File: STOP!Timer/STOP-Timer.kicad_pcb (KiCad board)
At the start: 2 copper layers, 4 parts, among them SW1 SW_Push_DPDT, U2 PEC11R-4230F-S0024, U3 PEC11R-4230F-S0024

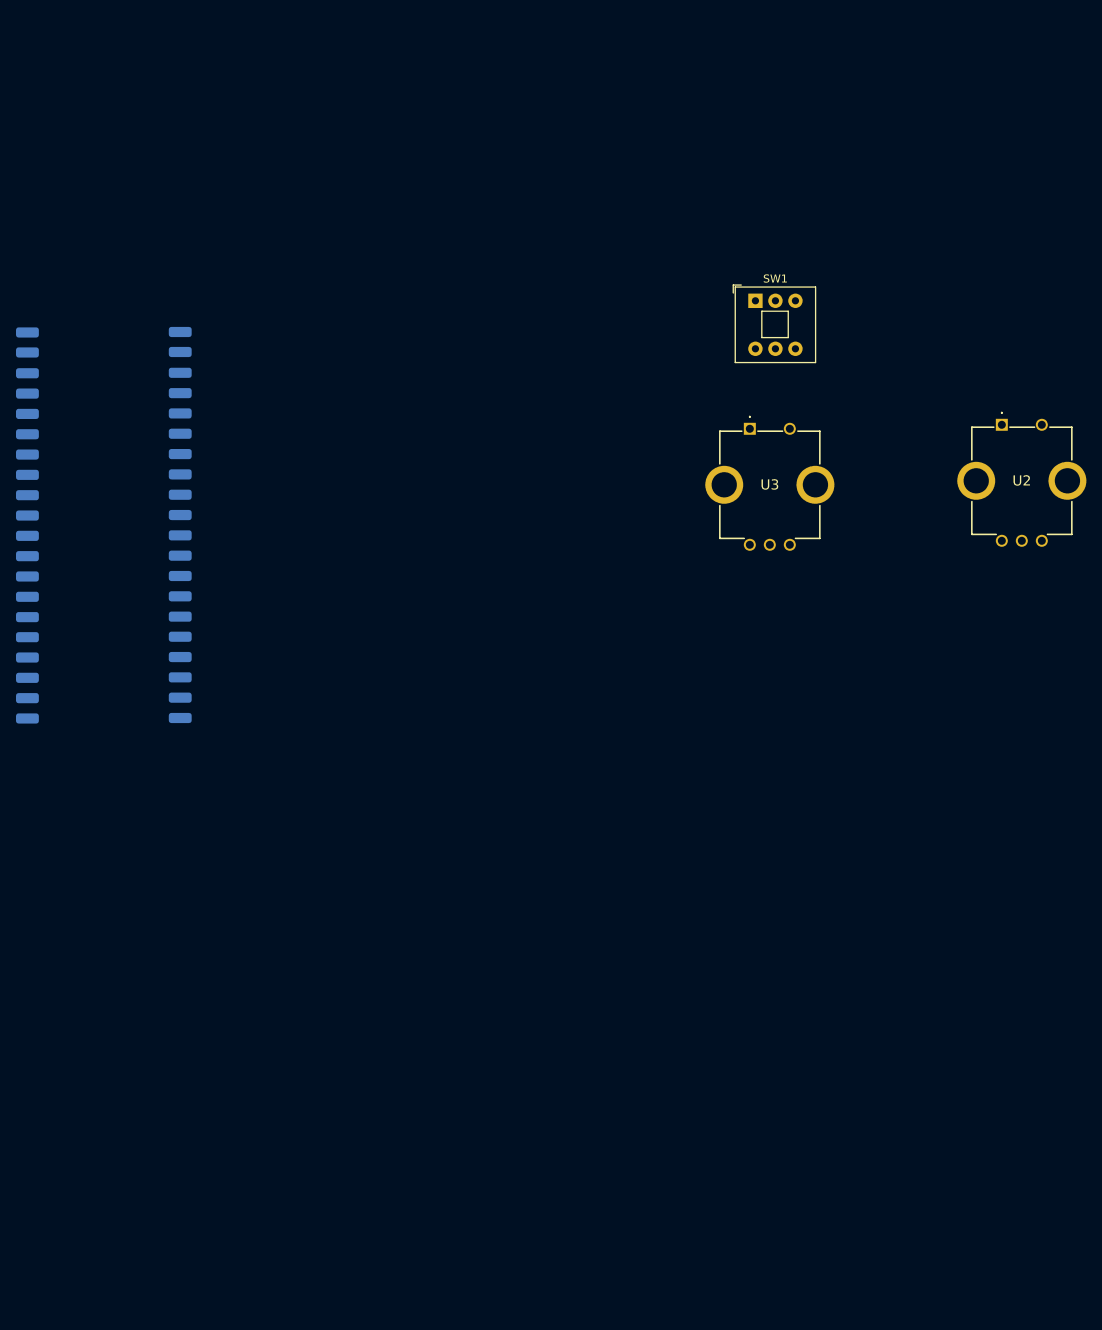
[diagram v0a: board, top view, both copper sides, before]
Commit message: Update Schematic
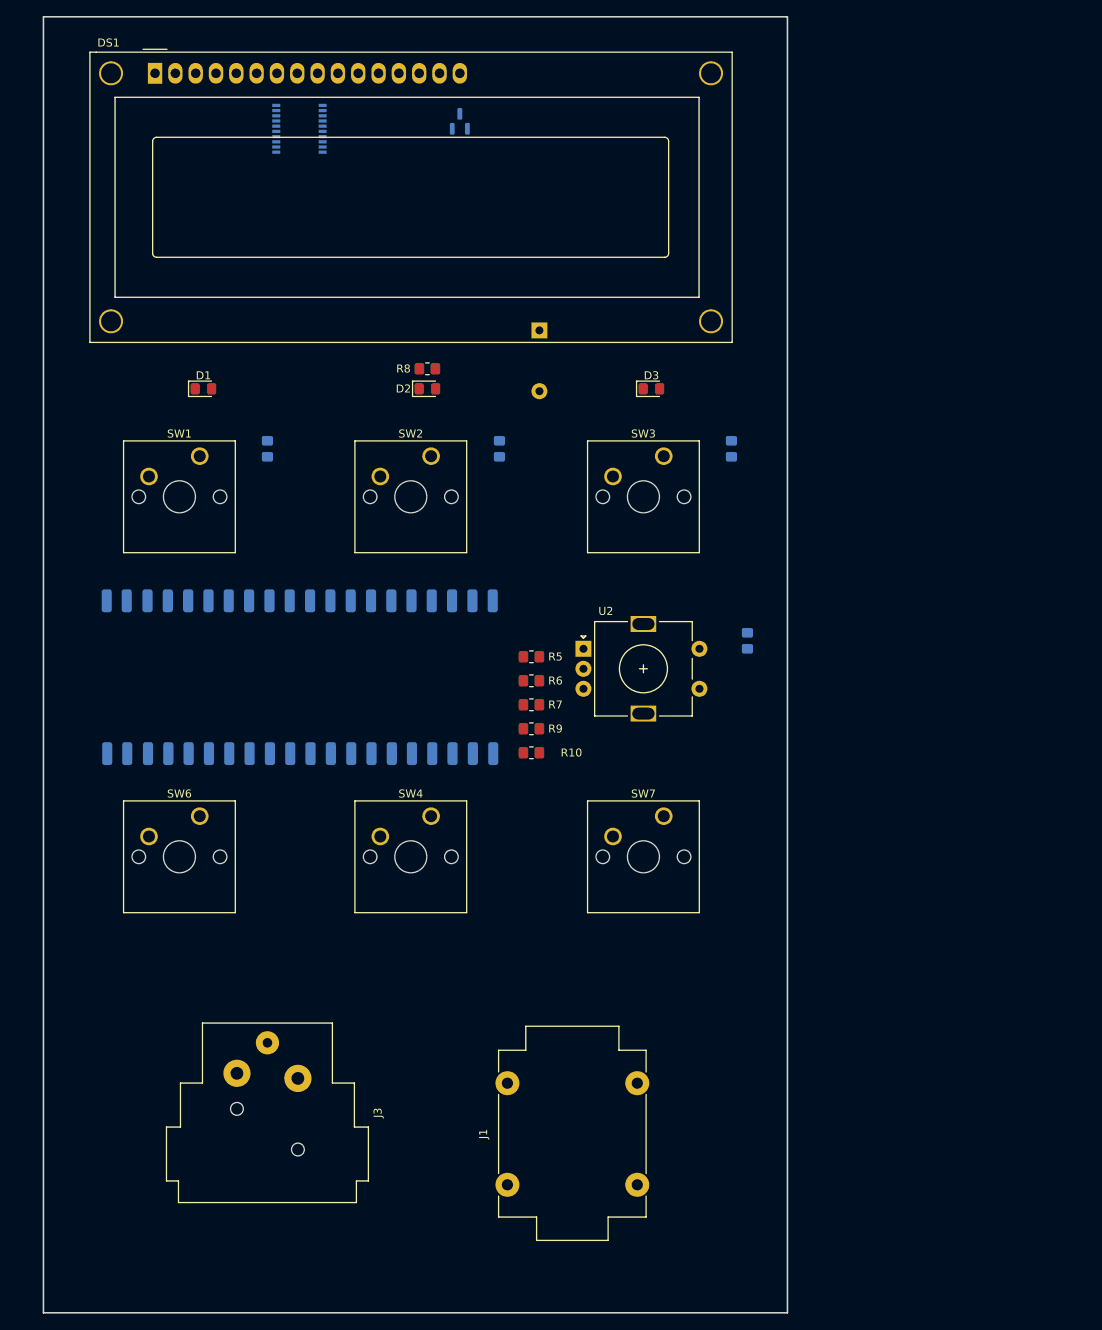
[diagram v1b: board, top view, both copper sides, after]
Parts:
- removed U3: PEC11R-4230F-S0024, project_footprints:PEC11R4225FS0012
- added BZ1: Buzzer, Buzzer_Beeper:Buzzer_12x9.5RM7.6, B.Cu at (115.0, 64.2)
- added D1: LED, LED_SMD:LED_0805_2012Metric_Pad1.15x1.40mm_HandSolder, F.Cu at (73.0, 71.5)
- added D2: LED, LED_SMD:LED_0805_2012Metric_Pad1.15x1.40mm_HandSolder, F.Cu at (101.0, 71.5)
- added D3: LED, LED_SMD:LED_0805_2012Metric_Pad1.15x1.40mm_HandSolder, F.Cu at (129.0, 71.5)
- added DS1: HY1602E, Display:WC1602A, F.Cu at (67.0, 32.1)
- added J1: Foot Switch Jack, Connector_Audio:Jack_6.35mm_Neutrik_NMJ4HCD2_Horizontal, F.Cu at (111.0, 171.0)
- added J3: XLR3, Connector_Audio:Jack_XLR_Neutrik_NC3FAAH-0_Horizontal, F.Cu at (84.8, 157.7)
- added Q1: AO3401A, Package_TO_SOT_SMD:SOT-23, B.Cu at (105.0, 38.1)
- added R10: 1k, Resistor_SMD:R_0805_2012Metric_Pad1.20x1.40mm_HandSolder, F.Cu at (114.0, 117.0)
- added R11: 1k, Resistor_SMD:R_0805_2012Metric_Pad1.20x1.40mm_HandSolder, B.Cu at (141.0, 103.0)
- added R2: 1k, Resistor_SMD:R_0805_2012Metric_Pad1.20x1.40mm_HandSolder, B.Cu at (81.0, 79.0)
- added R3: 1k, Resistor_SMD:R_0805_2012Metric_Pad1.20x1.40mm_HandSolder, B.Cu at (110.0, 79.0)
- added R4: 1k, Resistor_SMD:R_0805_2012Metric_Pad1.20x1.40mm_HandSolder, B.Cu at (139.0, 79.0)
- added R5: 1k, Resistor_SMD:R_0805_2012Metric_Pad1.20x1.40mm_HandSolder, F.Cu at (114.0, 105.0)
- added R6: 1k, Resistor_SMD:R_0805_2012Metric_Pad1.20x1.40mm_HandSolder, F.Cu at (114.0, 108.0)
- added R7: 1k, Resistor_SMD:R_0805_2012Metric_Pad1.20x1.40mm_HandSolder, F.Cu at (114.0, 111.0)
- added R8: R, Resistor_SMD:R_0805_2012Metric_Pad1.20x1.40mm_HandSolder, F.Cu at (101.0, 69.0)
- added R9: 1k, Resistor_SMD:R_0805_2012Metric_Pad1.20x1.40mm_HandSolder, F.Cu at (114.0, 114.0)
- added SW2: SW_Push, Button_Switch_Keyboard:SW_Cherry_MX_1.50u_PCB, F.Cu at (101.5, 79.9)
- added SW3: SW_Push, Button_Switch_Keyboard:SW_Cherry_MX_1.50u_PCB, F.Cu at (130.5, 79.9)
- added SW4: SW_Push, Button_Switch_Keyboard:SW_Cherry_MX_1.50u_PCB, F.Cu at (101.5, 124.9)
- added SW6: SW_Push, Button_Switch_Keyboard:SW_Cherry_MX_1.50u_PCB, F.Cu at (72.5, 124.9)
- added SW7: SW_Push, Button_Switch_Keyboard:SW_Cherry_MX_1.50u_PCB, F.Cu at (130.5, 124.9)
- added U4: PCF8574, Package_SO:SSOP-20_4.4x6.5mm_P0.65mm, B.Cu at (85.0, 39.0)
- SW1: value SW_Push_DPDT -> SW_Push; footprint Button_Switch_THT:SW_Push_2P2T_Toggle_CK_PVA2xxH4xxxxxxV2 -> Button_Switch_Keyboard:SW_Cherry_MX_1.50u_PCB
- U2: value PEC11R-4230F-S0024 -> EC11E18244AU; footprint project_footprints:PEC11R4225FS0012 -> Rotary_Encoder:RotaryEncoder_Alps_EC11E-Switch_Vertical_H20mm
- moved SW1 72.1 mm to (72.5, 79.9)
- moved U2 59.3 mm to (120.5, 104.0)
- moved U1 29.9 mm to (78.2, 106.5), turned to -90 degrees
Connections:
- SW1 pad 1: unconnected-(SW1-A-Pad1) -> TIME_SEL_1
- SW1 pad 2: unconnected-(SW1-B-Pad2) -> GND
- U1 pad 18: unconnected-(U1-GND-Pad18) -> GND
- U1 pad 23: unconnected-(U1-GND-Pad23) -> GND
- U1 pad 3: unconnected-(U1-GND-Pad3) -> GND
- U1 pad 38: unconnected-(U1-GND-Pad38) -> GND
- U1 pad 40: unconnected-(U1-VBUS-Pad40) -> VCC
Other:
- board outline added: 93 x 162 mm
